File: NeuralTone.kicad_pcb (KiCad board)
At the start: 2 copper layers, 85 parts, among them J1 Guitar, J2 5V@3A, J3 Headphones, J4 USB Port, J5 Line Out, J6 TF-01A, J7 RPi CM4Lite Compatible, J8 RPi CM4Lite Compatible, SW1 SW_Push, U1 LDLN025M33R, U2 CH224K, U3 MCP6022, U4 LDLN025M33R, U5 AP2151, U6 NAU8814YG, Y1 DSB211SDN 26MHz

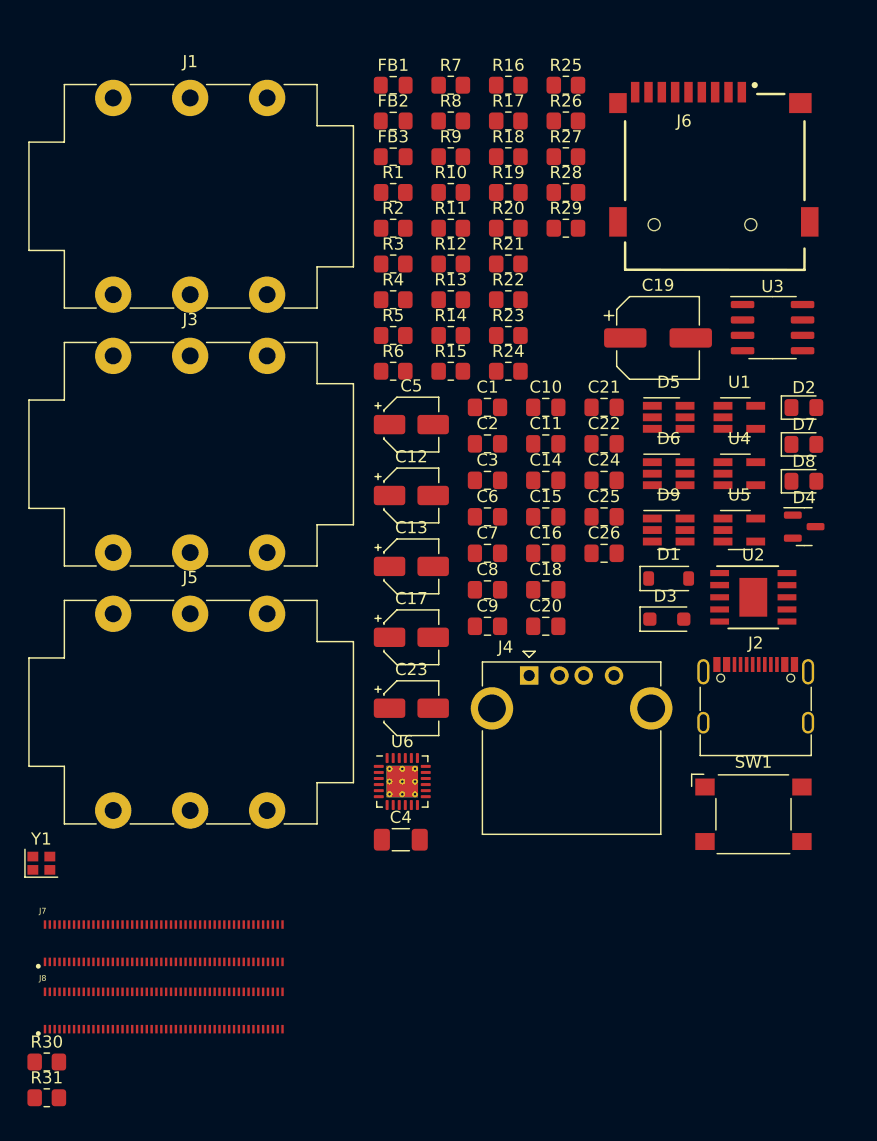
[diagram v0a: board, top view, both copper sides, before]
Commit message: cleanup and lcsc part numbers
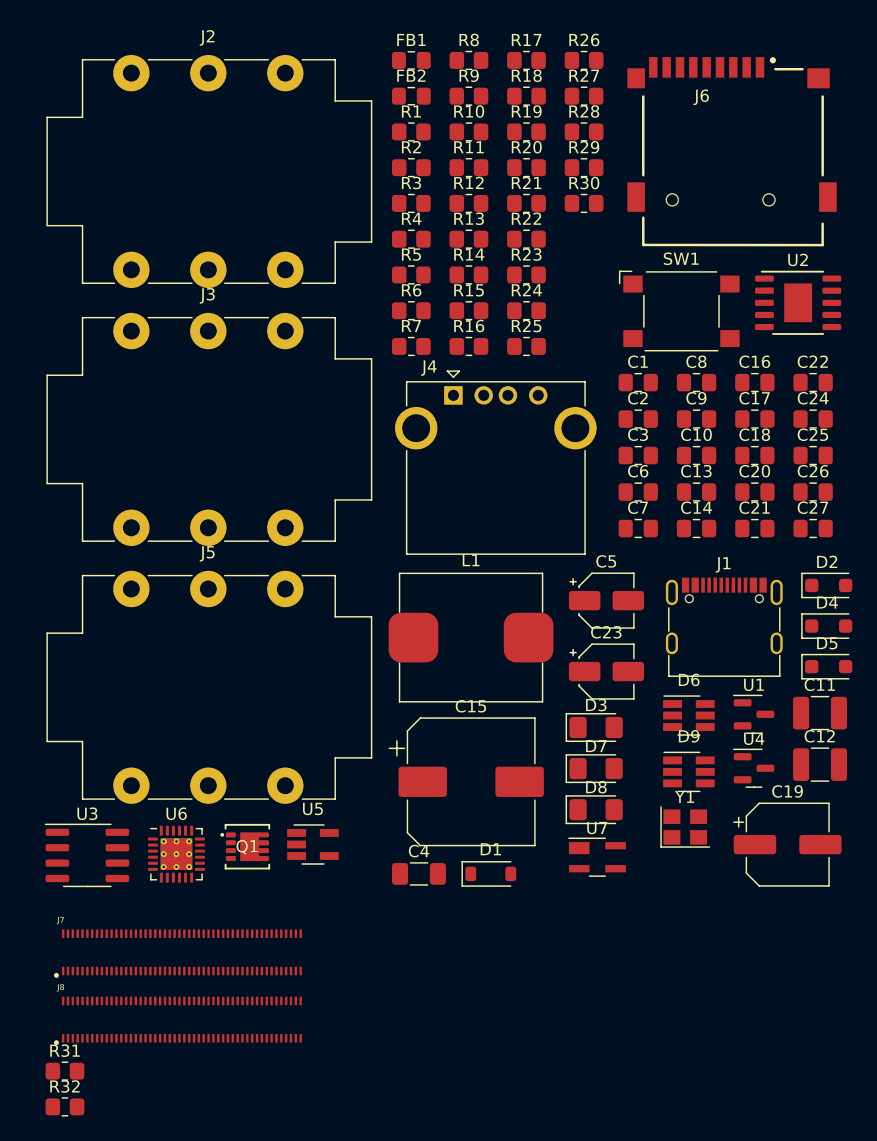
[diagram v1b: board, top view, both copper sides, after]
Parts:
- removed FB3: BLM21AG102SN1, Inductor_SMD:L_0805_2012Metric_Pad1.15x1.40mm_HandSolder
- added C27: 4.7u, Capacitor_SMD:C_0805_2012Metric_Pad1.18x1.45mm_HandSolder, F.Cu at (180.7, 87.5)
- added L1: 104CDMCCDS 4.7u, NeuralTone:104CDMCC_DS, F.Cu at (152.5, 96.5)
- added Q1: AON7421, NeuralTone:DMP2008UFG, F.Cu at (134.0, 113.8)
- added R32: 330, Resistor_SMD:R_0805_2012Metric_Pad1.20x1.40mm_HandSolder, F.Cu at (119.0, 135.2)
- added U7: DRTR5V0U2SR, Package_TO_SOT_SMD:SOT-143_Handsoldering, F.Cu at (162.9, 114.6)
- C10: value 10n -> 100n
- C11: value 10n -> 47u; footprint Capacitor_SMD:C_0805_2012Metric_Pad1.18x1.45mm_HandSolder -> Capacitor_SMD:C_1210_3225Metric_Pad1.33x2.70mm_HandSolder
- C12: value 22u -> 47u; footprint Capacitor_SMD:CP_Elec_4x5.4 -> Capacitor_SMD:C_1210_3225Metric_Pad1.33x2.70mm_HandSolder
- C13: value 22u -> 4.7u; footprint Capacitor_SMD:CP_Elec_4x5.4 -> Capacitor_SMD:C_0805_2012Metric_Pad1.18x1.45mm_HandSolder
- C15: value 4.7u -> 470u; footprint Capacitor_SMD:C_0805_2012Metric_Pad1.18x1.45mm_HandSolder -> Capacitor_SMD:CP_Elec_10x10
- C16, C24: value 100p -> 33p
- C17: value 22u -> 33p; footprint Capacitor_SMD:CP_Elec_4x5.4 -> Capacitor_SMD:C_0805_2012Metric_Pad1.18x1.45mm_HandSolder
- C19: footprint Capacitor_SMD:CP_Elec_6.3x5.8 -> Capacitor_SMD:CP_Elec_6.3x7.7
- C2, C6: value 4.7u -> 1u
- C23, C5: footprint Capacitor_SMD:CP_Elec_4x5.4 -> Capacitor_SMD:CP_Elec_4x5.3
- C25: value 470n -> 33p
- C26: value 4.7u -> 100n
- C8: value 470n -> 4.7u
- C9: value 470n -> 1u
- D2: value LED_Small -> SMF5.0A; footprint LED_SMD:LED_0805_2012Metric_Pad1.15x1.40mm_HandSolder -> Diode_SMD:D_SOD-123F
- D3: value SMF5.0A -> LED_Small; footprint Diode_SMD:D_SOD-123F -> LED_SMD:LED_1206_3216Metric_Pad1.42x1.75mm_HandSolder
- D4: value PESD5V2S2UT -> SMF5.0CA; footprint Package_TO_SOT_SMD:SOT-23 -> Diode_SMD:D_SOD-123F
- D5: value USBLC6-2P6 -> SMF5.0CA; footprint Package_TO_SOT_SMD:SOT-23-6_Handsoldering -> Diode_SMD:D_SOD-123F
- D7, D8: footprint LED_SMD:LED_0805_2012Metric_Pad1.15x1.40mm_HandSolder -> LED_SMD:LED_1206_3216Metric_Pad1.42x1.75mm_HandSolder
- FB2: value BLM21AG102SN1 -> BLM21PG220SN1
- J1: value Guitar -> USB C; footprint Connector_Audio:Jack_6.35mm_Neutrik_NMJ6HCD2_Horizontal -> Connector_USB:USB_C_Receptacle_G-Switch_GT-USB-7010ASV
- J2: value 5V@3A -> Guitar; footprint Connector_USB:USB_C_Receptacle_G-Switch_GT-USB-7010ASV -> Connector_Audio:Jack_6.35mm_Neutrik_NMJ6HCD2_Horizontal
- J7, J8: value RPi CM4Lite Compatible -> DF40HC(3.0)-100DS
- R10: value 10k -> 220m
- R11: value 2.2M -> 220m
- R12, R13: value 10k -> 1k
- R14, R3: value 10k -> 1.8k
- R22: value 22 -> 10k
- R23, R26: value 1k -> 22
- R24, R27: value 22 -> 1k
- R30: value 330 -> 22
- R4: value 10k -> 3.9k
- R5: value 1.8k -> 10k
- R6: value 3.9k -> 2.2M
- R7: value 100 -> 10k
- R8: value 2.2M -> 10k
- U1, U4: value LDLN025M33R -> AP2125N-3.3; footprint Package_TO_SOT_SMD:SOT-23-5_HandSoldering -> Package_TO_SOT_SMD:SOT-23
- Y1: value DSB211SDN 26MHz -> OT322512MJBA4SL; footprint Crystal:Crystal_SMD_2016-4Pin_2.0x1.6mm -> Crystal:Crystal_SMD_3225-4Pin_3.2x2.5mm
- moved R30 83.6 mm to (161.8, 60.7)
- moved J2 73.6 mm to (124.5, 49.9)
- moved U3 71.4 mm to (120.8, 114.5)
- moved J1 66.9 mm to (173.4, 95.9)
- moved Y1 53.2 mm to (170.2, 112.1)
- moved U5 43.7 mm to (139.4, 113.6)
- moved C19 43.2 mm to (178.6, 113.6)
- moved SW1 41.9 mm to (169.8, 69.6)
- moved C12 40.4 mm to (181.3, 107.0)
- moved C17 33.6 mm to (175.9, 78.5)
- moved D8 32.1 mm to (162.8, 110.7)
- moved D7 31.8 mm to (162.8, 107.3)
- moved C11 31.7 mm to (181.3, 102.7)
- moved D1 28.4 mm to (154.1, 116.0)
- moved U2 24.6 mm to (179.5, 68.9)
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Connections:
- C10 pad 1: /VBUS -> GND
- C10 pad 2: GND -> +3V3A_B
- C11 pad 1: +5V -> Net-(C11-Pad1)
- C12 pad 1: +5V -> Net-(C12-Pad1)
- C13 pad 1: +5V -> +3V3A_C
- C15 pad 1: +3V3A_C -> /HEADPHONES
- C15 pad 2: GND -> Net-(C15-Pad2)
- C16 pad 1: Net-(C16-Pad1) -> GND
- C16 pad 2: GND -> Net-(C15-Pad2)
- C17 pad 1: /HEADPHONES -> GND
- C17 pad 2: Net-(C16-Pad1) -> Net-(C17-Pad2)
- C2 pad 1: +3V3A_B -> +5V
- C25 pad 1: +3V3 -> GND
- C25 pad 2: GND -> Net-(C25-Pad2)
- C3 pad 1: +5V -> +3V3A_B
- C5 pad 2: Net-(C5-Pad2) -> CODEC_AUX
- C6 pad 1: +3V3A_C -> +5V
- C7 pad 1: +5V -> +3V3A_C
- C9 pad 1: GND -> Net-(Q1-D)
- C9 pad 2: +3V3A_B -> Net-(Q1-G)
- D2 pad 1: Net-(D2-K) -> /VBUS
- D2 pad 2: Net-(D2-A) -> GND
- D3 pad 1: /VBUS -> GND
- D3 pad 2: GND -> Net-(D3-A)
- D4 pad 1: Net-(C16-Pad1) -> GND
- D4 pad 2: Net-(C23-Pad2) -> Net-(C17-Pad2)
- D5 pad 1: USBD+ -> GND
- D5 pad 2: GND -> Net-(C25-Pad2)
- FB1 pad 1: /VBUS -> Net-(C15-Pad2)
- FB1 pad 2: +5V -> Net-(C17-Pad2)
- FB2 pad 1: Net-(C16-Pad1) -> Net-(C23-Pad2)
- FB2 pad 2: Net-(FB2-Pad2) -> Net-(C25-Pad2)
- J3 pad R: Net-(FB2-Pad2) -> Net-(C17-Pad2)
- J3 pad T: Net-(FB2-Pad2) -> Net-(C17-Pad2)
- J4 pad 2: Net-(J4-D-) -> USBD-
- J4 pad 3: Net-(J4-D+) -> USBD+
- J5 pad R: Net-(FB3-Pad2) -> Net-(C25-Pad2)
- J5 pad T: Net-(FB3-Pad2) -> Net-(C25-Pad2)
- R10 pad 1: GND -> Net-(Q1-D)
- R10 pad 2: Net-(C5-Pad2) -> Net-(C11-Pad1)
- R11 pad 1: Net-(U3A--) -> +5V
- R11 pad 2: Net-(U3B-+) -> Net-(C12-Pad1)
- R12 pad 1: Net-(U3A-+) -> +5V
- R12 pad 2: +3V3A_B -> Net-(D3-A)
- R13 pad 1: +5V -> Net-(Q1-G)
- R13 pad 2: Net-(U4-EN) -> /PG
- R14 pad 1: GND -> Net-(C15-Pad2)
- R14 pad 2: Net-(U3A-+) -> GND
- R2 pad 1: +5V -> Net-(U2-CFG1)
- R2 pad 2: Net-(U1-EN) -> /VDD
- R21 pad 1: GND -> Net-(C23-Pad2)
- R21 pad 2: Net-(U6-CSb/GPIO) -> GND
- R22 pad 1: SD_DAT2 -> GND
- R22 pad 2: Net-(J6-DAT2) -> Net-(U6-CSb/GPIO)
- R23 pad 1: LED_STAT_1 -> SD_DAT2
- R23 pad 2: Net-(D7-A) -> Net-(J6-DAT2)
- R24 pad 1: SD_DAT3 -> LED_STAT_1
- R24 pad 2: Net-(J6-DAT3/CD) -> Net-(D7-A)
- R25 pad 1: SD_CMD -> SD_DAT3
- R25 pad 2: Net-(J6-CMD) -> Net-(J6-DAT3/CD)
- R26 pad 1: LED_STAT_2 -> SD_CMD
- R26 pad 2: Net-(D8-A) -> Net-(J6-CMD)
- R27 pad 1: SD_CLK -> LED_STAT_2
- R27 pad 2: Net-(J6-CLK) -> Net-(D8-A)
- R28 pad 1: SD_DAT0 -> SD_CLK
- R28 pad 2: Net-(J6-DAT0) -> Net-(J6-CLK)
- R29 pad 1: SD_DAT1 -> SD_DAT0
- R29 pad 2: Net-(J6-DAT1) -> Net-(J6-DAT0)
- R3 pad 1: /VBUS -> Net-(J2-PadT)
- R3 pad 2: Net-(U2-VBUS) -> Net-(D1-A)
- R30 pad 1: I2C_SCL -> SD_DAT1
- R30 pad 2: Net-(J7-GPIO3) -> Net-(J6-DAT1)
- R31 pad 1: I2C_SDA -> I2C_SCL
- R31 pad 2: Net-(J7-GPIO2) -> Net-(J7-GPIO3)
- R4 pad 1: Net-(U2-CFG1) -> Net-(D1-A)
- R4 pad 2: /VDD -> Net-(C4-Pad1)
- R5 pad 1: Net-(J1-PadT) -> GND
- R5 pad 2: Net-(D1-A) -> CODEC_AUX
- R6 pad 1: Net-(D1-A) -> Net-(U3A--)
- R6 pad 2: Net-(C4-Pad1) -> Net-(U3B-+)
- R7 pad 1: Net-(C5-Pad2) -> Net-(U3A-+)
- R7 pad 2: CODEC_AUX -> +3V3A_B
- R8 pad 1: Net-(C4-Pad1) -> GND
- R8 pad 2: GND -> Net-(U3A-+)
- R9 pad 1: Net-(D2-A) -> /VBUS
- R9 pad 2: /VDD -> Net-(Q1-G)
- U1 pad 1: +5V -> GND
- U1 pad 2: GND -> +3V3A_B
- U1 pad 3: Net-(U1-EN) -> +5V
- U2 pad 10: Net-(D2-K) -> /PG
- U2 pad 4: Net-(U2-DP) -> Net-(U2-DM)
- U2 pad 6: Net-(J2-CC2) -> Net-(J1-CC2)
- U2 pad 7: Net-(J2-CC1) -> Net-(J1-CC1)
- U2 pad 8: Net-(U2-VBUS) -> unconnected-(U2-VBUS-Pad8)
- U4 pad 1: +5V -> GND
- U4 pad 2: GND -> +3V3A_C
- U4 pad 3: Net-(U4-EN) -> +5V
- Y1 pad 1: GND -> unconnected-(Y1-Pad1)
